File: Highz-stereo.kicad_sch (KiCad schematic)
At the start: 83 parts, among them J1 Conn_01x01_Female, J10 Conn_01x01_Female, J11 Conn_01x01_Female, J12 Conn_01x01_Female, J13 potmeter ground B, J14 Potmeter ground A, J16 Conn_01x01_Female, J17 Conn_01x01_Female, J18 Conn_01x01_Female, J19 Conn_01x01_Female, J1A1 Conn_01x01_Female, J2 Conn_01x01_Female, J20 Conn_01x01_Female, J3 Potmeter ground A, J3A1 Conn_01x01_Female, J4 Conn_01x01_Female, J5 Conn_01x01_Female, J6 potmeter ground B, J6A1 Conn_01x01_Female, J7 Conn_01x01_Female, J8 Conn_01x01_Female, J9 Conn_01x01_Female, U2 OPA1679

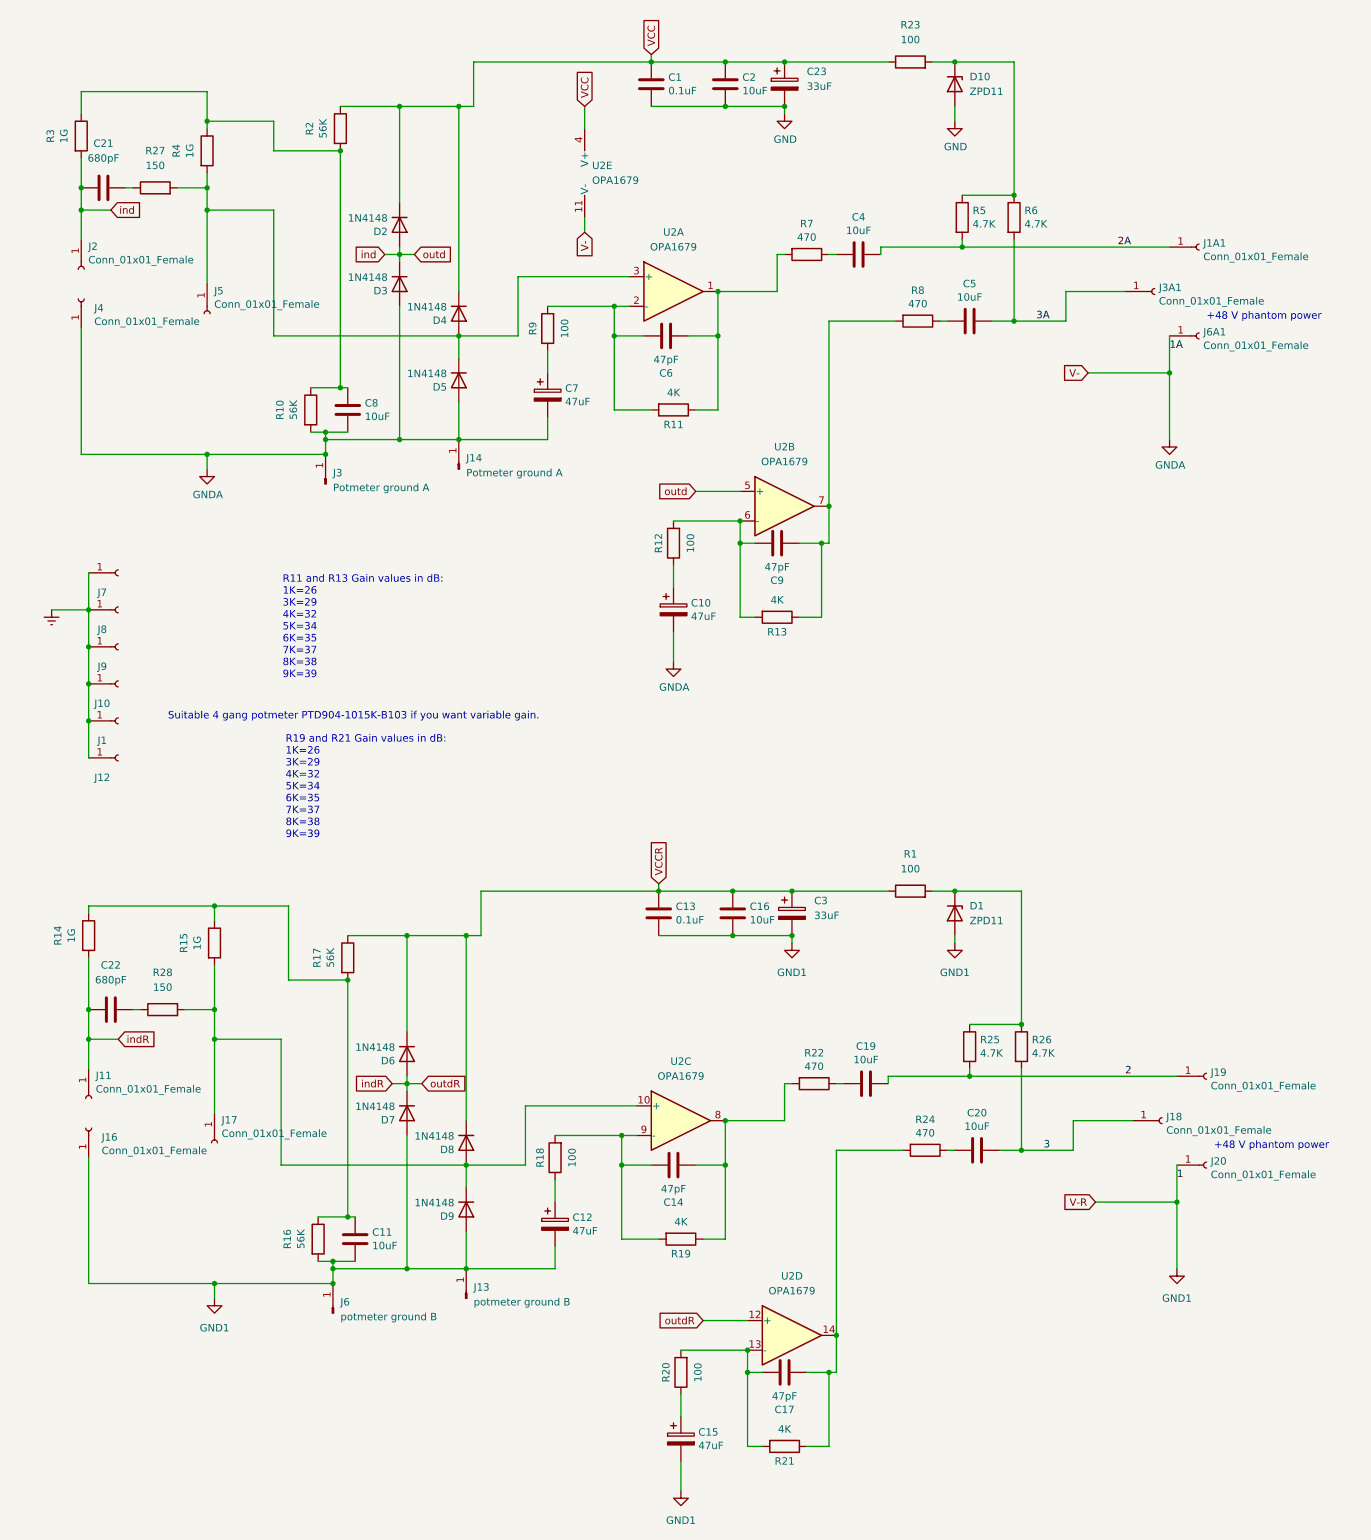
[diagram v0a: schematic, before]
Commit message: Add files via upload
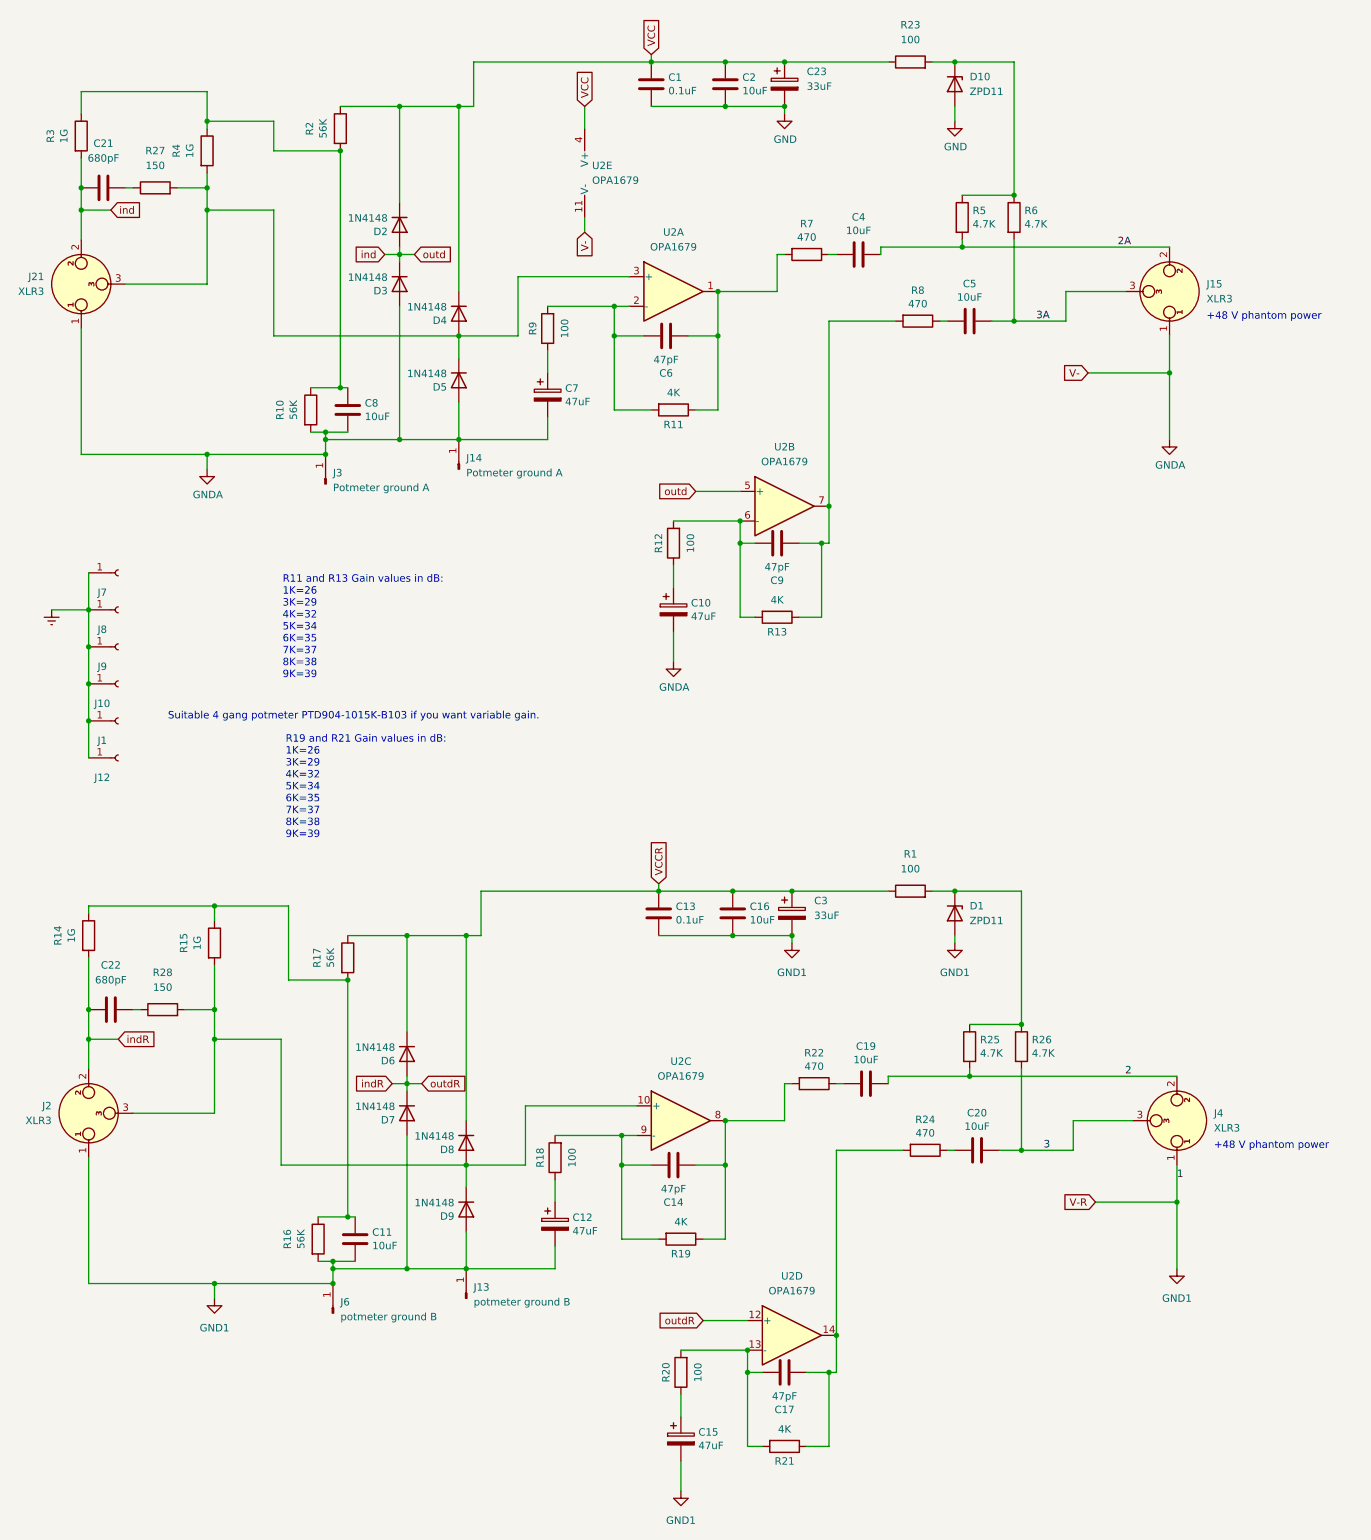
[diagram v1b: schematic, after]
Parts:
- removed J11, J16, J17, J18, J19, J1A1, J2, J20, J3A1, J4, J5, J6A1: Conn_01x01_Female, MountingHole:MountingHole_2.2mm_M2_ISO7380_Pad, symbol double-gain-rescue:Conn_01x01_Female-Connector
- added J15, J2, J21, J4: XLR3, Connector_Wire:SolderWire-0.25sqmm_1x03_P4.5mm_D0.65mm_OD2mm, symbol Connector_Audio:XLR3
- C1, C13: mfr (none) -> TAP104K050SCS
- C10, C12, C15, C7: mfr (none) -> ECA-2AM470BJ
- C11, C16, C19, C2, C20, C4, C5, C8: mfr (none) -> B32522C0106K000
- C14, C17, C6, C9: mfr (none) -> FKP2O100471D00KSSD
- C21, C22: mfr (none) -> FKP2D006801D00KSSD
- C23, C3: mfr (none) -> 860010672011
- D1, D10: mfr (none) -> ZPD11
- D2, D3, D4, D5, D6, D7, D8, D9: mfr (none) -> 1N4148
- R1, R12, R18, R20, R23, R9: mfr (none) -> YR1B100RCC
- R10, R16, R17, R2: mfr (none) -> RNMF14FTC56K0
- R11, R13, R19, R21: mfr (none) -> RN60D4001FRE6
- R14, R15, R3, R4: mfr (none) -> RGP0207CHK1G0
- R22, R24, R7, R8: mfr (none) -> MFR-25FTE52-470R
- R25, R26, R5, R6: mfr (none) -> RNMF14FTC4K70
- R27, R28: mfr (none) -> RNF14FTD150R
- U2: mfr (none) -> OPA1679IDR
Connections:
- net 2: now also J4.2
- net 2A: now also J15.2
- net 3: now also J4.3
- net 3A: now also J15.3
- net GND1: now also J2.1, J4.1
- net GNDA: now also J15.1, J21.1
- net ind: now also J21.2
- net indR: now also J2.2
- net at D4.2 (A), D5.1 (K), R27.2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: now also J21.3
- net at D8.2 (A), D9.1 (K), R15.2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: now also J2.3
